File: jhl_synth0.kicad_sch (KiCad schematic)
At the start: 45 parts, among them J1 Conn_01x01, J10 Conn_01x04, J11 Conn_01x01, J12 Conn_01x01, J13 Conn_01x01, J14 Conn_01x01, J15 Conn_01x01, J16 Conn_01x01, J17 Conn_01x01, J18 Conn_01x04, J19 Conn_01x01, J2 USB_B_Micro, J20 Conn_02x05_Odd_Even, J21 Conn_01x01, J22 Conn_01x01, J23 Conn_01x01, J24 Conn_01x01, J25 Conn_01x01, J26 Conn_01x01, J27 Conn_01x04, J28 Conn_01x01, J29 Conn_01x01, J3 Conn_01x01, J30 Conn_02x05_Odd_Even, J35 Conn_01x04, J36 Conn_01x03, J4 Conn_01x01, J5 Conn_01x08, J6 Conn_01x08, J7 Conn_01x04, J8 Conn_01x04, J9 Conn_01x04, U1 YAAJ_BlackPill, U2 YAAJ_BluePill

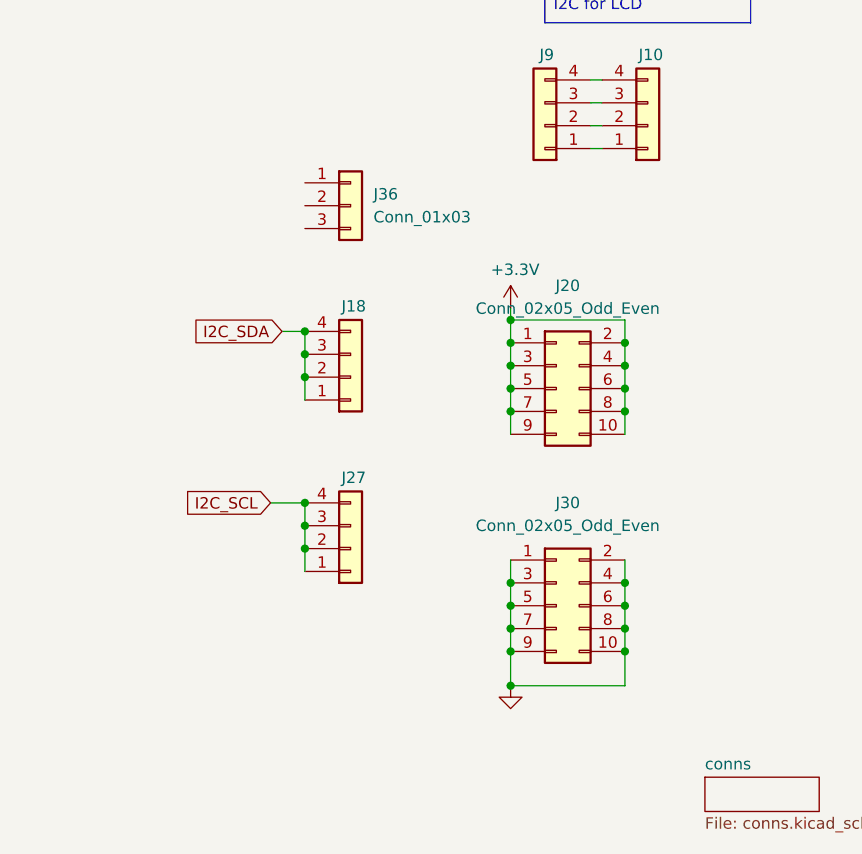
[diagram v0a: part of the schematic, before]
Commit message: 更新
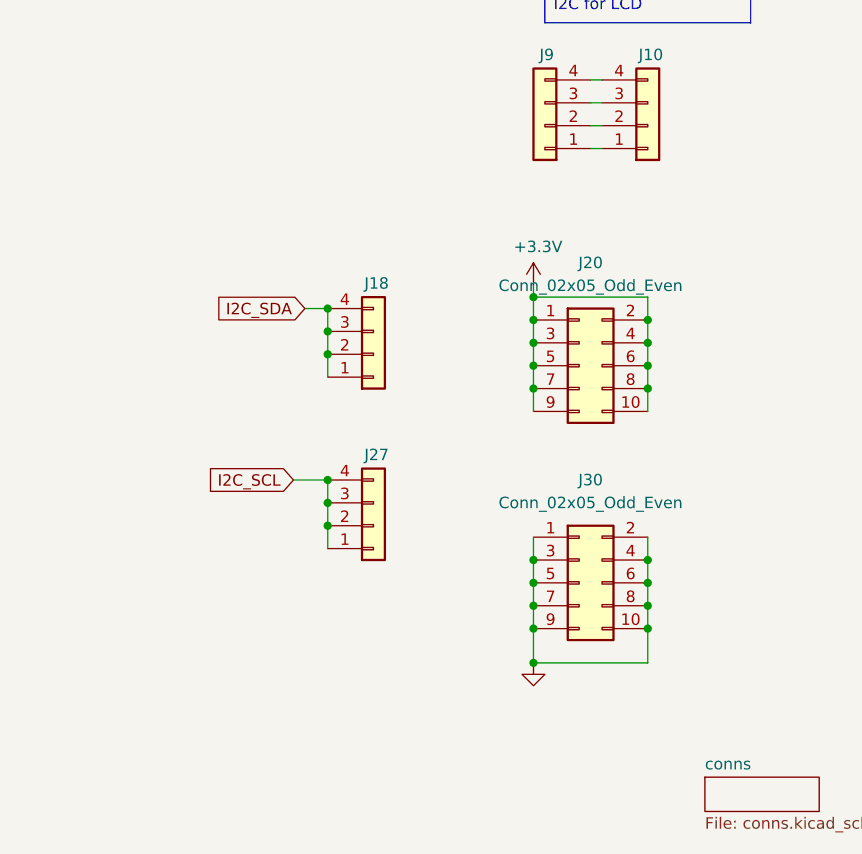
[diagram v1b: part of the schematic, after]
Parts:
- removed J36: Conn_01x03, Connector_PinHeader_2.54mm:PinHeader_1x03_P2.54mm_Vertical, symbol Connector_Generic:Conn_01x03
- J1, J3, J4: now left out of the parts list
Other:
- moved on the sheet: J18, J20, J27, J30
